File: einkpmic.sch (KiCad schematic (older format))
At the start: 42 parts

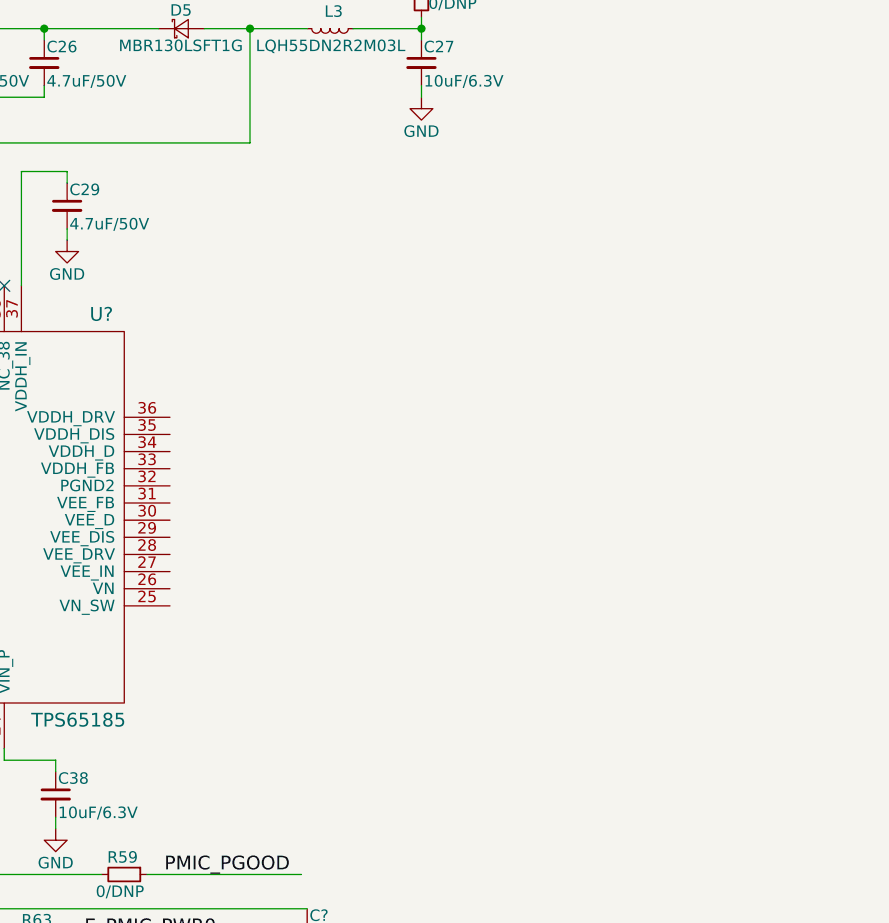
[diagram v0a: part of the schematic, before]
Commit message: update sch
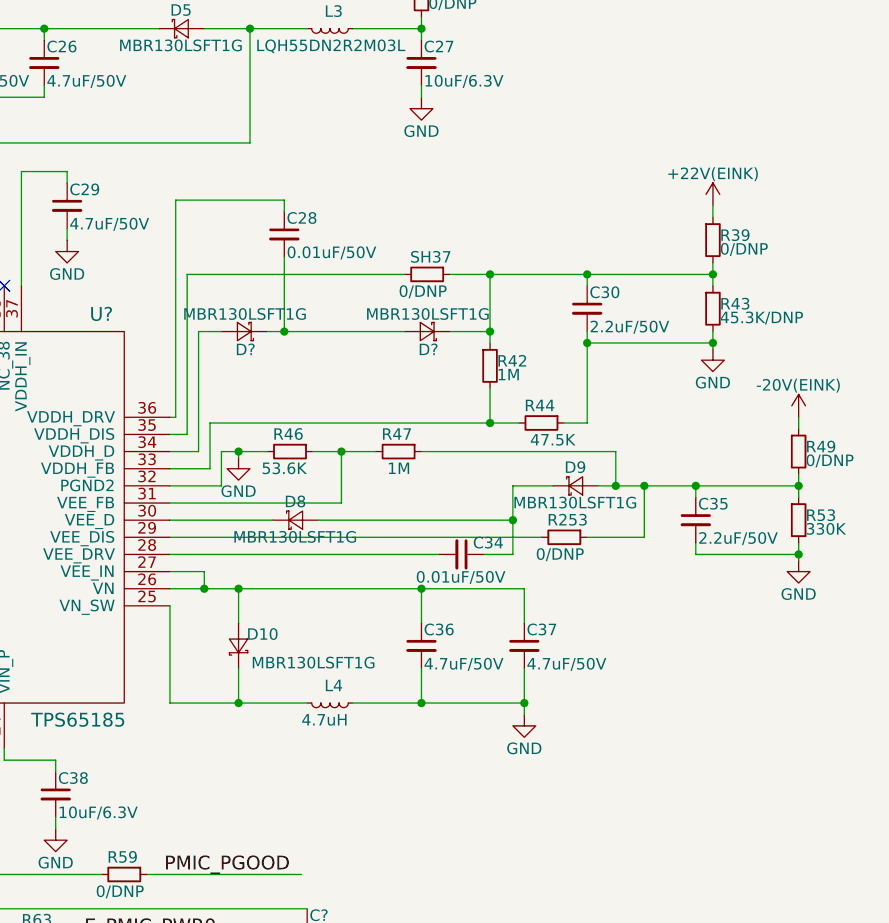
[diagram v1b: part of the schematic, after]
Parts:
- added C28, C34: 0.01uF/50V, symbol C_Small
- added C30, C35: 2.2uF/50V, symbol C_Small
- added C36, C37: 4.7uF/50V, symbol C_Small
- added D10, D8, D9, D? (x2): MBR130LSFT1G, symbol D_Schottky_Small
- added L4: 4.7uH, symbol L_Small
- added R253, R39, R49, SH37: 0/DNP, symbol R_Small
- added R42, R47: 1M, symbol R_Small
- added R43: 45.3K/DNP, symbol R_Small
- added R44: 47.5K, symbol R_Small
- added R46: 53.6K, symbol R_Small
- added R53: 330K, symbol R_Small
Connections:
- net labels added: +22V(EINK), -20V(EINK)
- wire segments 130 -> 193
